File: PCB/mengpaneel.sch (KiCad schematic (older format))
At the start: 296 parts, among them IC1 MAX7219CNG+, IC10 STM32F411CEU7, IC11 AD5204BRUZ10-REEL7, IC12 LTC3631EMS8E#TRPBF, IC13 LMV321AUIDBVR, IC2 MAX7219CNG+, IC3 MTCH6301-I_ML, IC4 LTC3121EDE#PBF, IC5 AD5204BRUZ10-REEL7, IC6 AD5204BRUZ10-REEL7, IC7 LM3480IM3-3.3_NOPB, IC8 AD5204BRUZ10-REEL7, IC9 AD5204BRUZ10-REEL7, J1 UJ2-MIBH-G-SMT-TR, J2 Screw_Terminal_01x03, J3 Screw_Terminal_01x14, J4 SJ-63053A, J5 SJ-63053A, J6 SJ-63053A, J7 SJ-63053A, SW1 SW_Push, SW2 SW_DPDT_x2, SW3 SW_DPST_x2, SW4 SW_DPST_x2, U11 Touchpad_mp, U13 Touchpad_mp_LR, U14 Touchpad_mp, U15 Touchpad_mp, U16 Touchpad_mp, U17 Touchpad_mp, U2 Touchpad_mp, U3 Touchpad_mp, U4 Touchpad_mp, U5 LM324N, U6 Touchpad_mp, U7 LM324N, U8 Touchpad_mp, Y1 8MHz

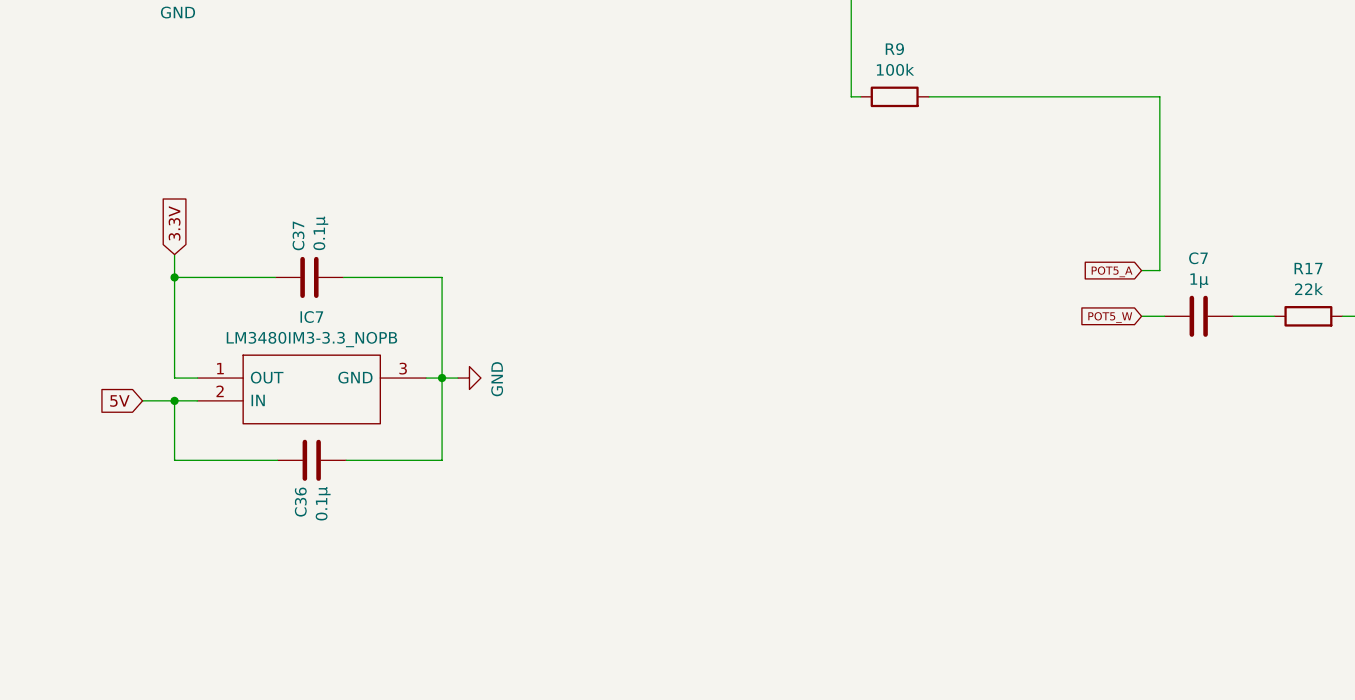
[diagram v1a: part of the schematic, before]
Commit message: Kleine foutjes nog aangepast.
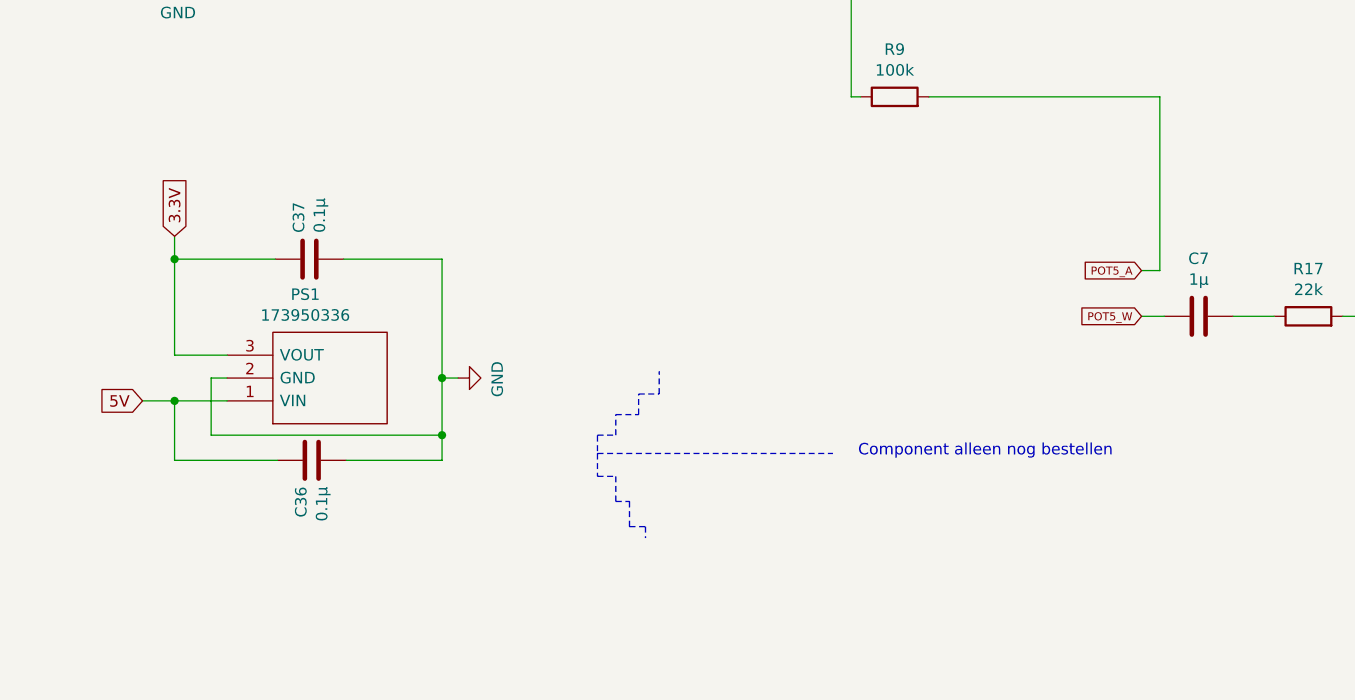
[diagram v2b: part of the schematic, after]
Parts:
- removed IC7: LM3480IM3-3.3_NOPB, LM3480IM3-3.3_NOPB:SOT95P237X112-3N, symbol mengpaneel-rescue:LM3480IM3-3.3_NOPB-LM3480IM3-3.3_NOPB
- added PS1: 173950336, 173950336:173950336, symbol 173950336:173950336
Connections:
- net 3.3V: now also PS1.3 (VOUT)
- net 5V: now also PS1.1 (VIN)
- net GND: now also PS1.2 (GND)
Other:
- note added: "Component alleen nog bestellen"
- moved on the sheet: C37
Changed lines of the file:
@@
 Wire Wire Line
 	15280 15050 15680 15050
-Connection ~ 16840 17500
-Wire Wire Line
-	16840 17500 16840 17400
-Wire Wire Line
-	18010 17500 18010 17940
-Wire Wire Line
-	17580 17500 18010 17500
-Wire Wire Line
-	16840 17500 17280 17500
-Wire Wire Line
-	16840 17940 16840 17500
-Wire Wire Line
-	16940 17940 16840 17940
+Wire Wire Line
+	16840 17420 16840 17320
+Wire Wire Line
+	17580 17420 18010 17420
+Wire Wire Line
+	16840 17420 17280 17420
 Wire Wire Line
 	18010 17940 18080 17940
-Connection ~ 18010 17940
-Wire Wire Line
-	18010 18300 18010 17940
+Wire Wire Line
+	18010 18300 18010 18190
 Wire Wire Line
 	17590 18300 18010 18300
 Wire Wire Line
-	16840 18040 16940 18040
-Wire Wire Line
 	16840 18300 17290 18300
 Wire Wire Line
 	16840 18040 16840 18300
-Wire Wire Line
-	17940 17940 18010 17940
-$Comp
-L mengpaneel-rescue:LM3480IM3-3.3_NOPB-LM3480IM3-3.3_NOPB IC7
-U 1 1 60ABB371
-P 16940 17940
-F 0 "IC7" H 17440 18205 50  0000 C CNN
-F 1 "LM3480IM3-3.3_NOPB" H 17440 18114 50  0000 C CNN
-F 2 "LM3480IM3-3.3_NOPB:SOT95P237X112-3N" H 17790 18040 50  0001 L CNN
-F 3 "http://www.ti.com/lit/ds/symlink/lm3480.pdf" H 17790 17940 50  0001 L CNN
-F 4 "100 mA, SOT-23, Quasi Low-Dropout Linear Voltage Regulator" H 17790 17840 50  0001 L CNN "Description"
-F 5 "1.12" H 17790 17740 50  0001 L CNN "Height"
-F 6 "926-LM3480IM33.3NOPB" H 17790 17640 50  0001 L CNN "Mouser Part Number"
-F 7 "https://www.mouser.co.uk/ProductDetail/Texas-Instruments/LM3480IM3-33-NOPB/?qs=X1J7HmVL2ZHWj012nPURIw%3D%3D" H 17790 17540 50  0001 L CNN "Mouser Price/Stock"
-F 8 "Texas Instruments" H 17790 17440 50  0001 L CNN "Manufacturer_Name"
-F 9 "LM3480IM3-3.3/NOPB" H 17790 17340 50  0001 L CNN "Manufacturer_Part_Number"
-	1    16940 17940
-	1    0    0    -1
-$EndComp
 $Comp
 L Device:C C36
@@
 L Device:C C37
 U 1 1 6062EFEB
-P 17430 17500
-F 0 "C37" H 17545 17546 50  0000 L CNN
-F 1 "0.1µ" H 17545 17455 50  0000 L CNN
-F 2 "06031C104K4Z2A:CAPC1608X90N" H 17468 17350 50  0001 C CNN
-F 3 "~" H 17430 17500 50  0001 C CNN
-	1    17430 17500
+P 17430 17420
+F 0 "C37" H 17545 17466 50  0000 L CNN
+F 1 "0.1µ" H 17545 17375 50  0000 L CNN
+F 2 "06031C104K4Z2A:CAPC1608X90N" H 17468 17270 50  0001 C CNN
+F 3 "~" H 17430 17420 50  0001 C CNN
+	1    17430 17420
 	0    -1   -1   0
 $EndComp
@@
 	0    -1   1    0
 $EndComp
-Text GLabel 16840 17400 1    50   Input ~ 0
+Text GLabel 16840 17320 1    50   Input ~ 0
 3.3V
 $Comp
@@
 NoConn ~ 7130 10900
 NoConn ~ 7130 11000
+Wire Notes Line
+	18690 18270 19720 18270
+Wire Notes Line
+	18690 18370 18770 18370
+Wire Notes Line
+	18770 18370 18770 18480
+Wire Notes Line
+	18770 18480 18830 18480
+Wire Notes Line
+	18830 18590 18900 18590
+Wire Notes Line
+	18690 18270 18690 18370
+Wire Notes Line
+	18830 18480 18830 18590
+Wire Notes Line
+	18900 18590 18900 18640
+Wire Notes Line
+	18690 18260 18690 18190
+Wire Notes Line
+	18690 18190 18770 18190
+Wire Notes Line
+	18770 18190 18770 18100
+Wire Notes Line
+	18770 18100 18870 18100
+Wire Notes Line
+	18870 18100 18870 18010
+Wire Notes Line
+	18870 18010 18960 18010
+Wire Notes Line
+	18960 18010 18960 17910
+Text Notes 19830 18290 0    50   ~ 0
+Component alleen nog bestellen
+$Comp
+L 173950336:173950336 PS1
+U 1 1 60F2F6D3
+P 17070 18040
+F 0 "PS1" H 17412 17575 50  0000 C CNN
+F 1 "173950336" H 17412 17666 50  0000 C CNN
+F 2 "173950336:173950336" H 17820 18140 50  0001 L CNN
+F 3 "https://componentsearchengine.com/Datasheets/2/173950336.pdf" H 17820 18040 50  0001 L CNN
+F 4 "WURTH ELEKTRONIK - 173950336 - DC/DC Converter, 1 Output, 1.65 W, 3.3 V, 500 mA, MagI3C FDSM Series" H 17820 17940 50  0001 L CNN "Description"
+F 5 "10.2" H 17820 17840 50  0001 L CNN "Height"
+F 6 "710-173950336" H 17820 17740 50  0001 L CNN "Mouser Part Number"
+F 7 "https://www.mouser.co.uk/ProductDetail/Wurth-Elektronik/173950336?qs=d0WKAl%252BL4KZw6hIvUkPbpg%3D%3D" H 17820 17640 50  0001 L CNN "Mouser Price/Stock"
+F 8 "Wurth Elektronik" H 17820 17540 50  0001 L CNN "Manufacturer_Name"
+F 9 "173950336" H 17820 17440 50  0001 L CNN "Manufacturer_Part_Number"
+	1    17070 18040
+	1    0    0    1
+$EndComp
+Wire Wire Line
+	16840 18040 17070 18040
+Wire Wire Line
+	17070 17840 16840 17840
+Connection ~ 16840 17420
+Wire Wire Line
+	17070 17940 17000 17940
+Wire Wire Line
+	17000 17940 17000 18190
+Wire Wire Line
+	17000 18190 18010 18190
+Connection ~ 18010 18190
+Wire Wire Line
+	18010 18190 18010 17940
+Wire Wire Line
+	18010 17420 18010 17940
+Connection ~ 18010 17940
+Wire Wire Line
+	16840 17420 16840 17840
 $EndSCHEMATC
